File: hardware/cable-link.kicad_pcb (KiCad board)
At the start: 4 copper layers, 50 x 50 mm, 58 parts, among them J1 USB_C_Receptacle_USB2.0, J2 Conn_01x02, J3 GBA-LINK, J4 SWD, Q1 BSS138, Q2 BSS138, Q3 BSS138, Q4 BSS138, U1 NCP1117-3.3_SOT223, U2 RP2040, U3 ATECC608A-MAHDA, U4 W25Q128JVS, Y1 12mhz

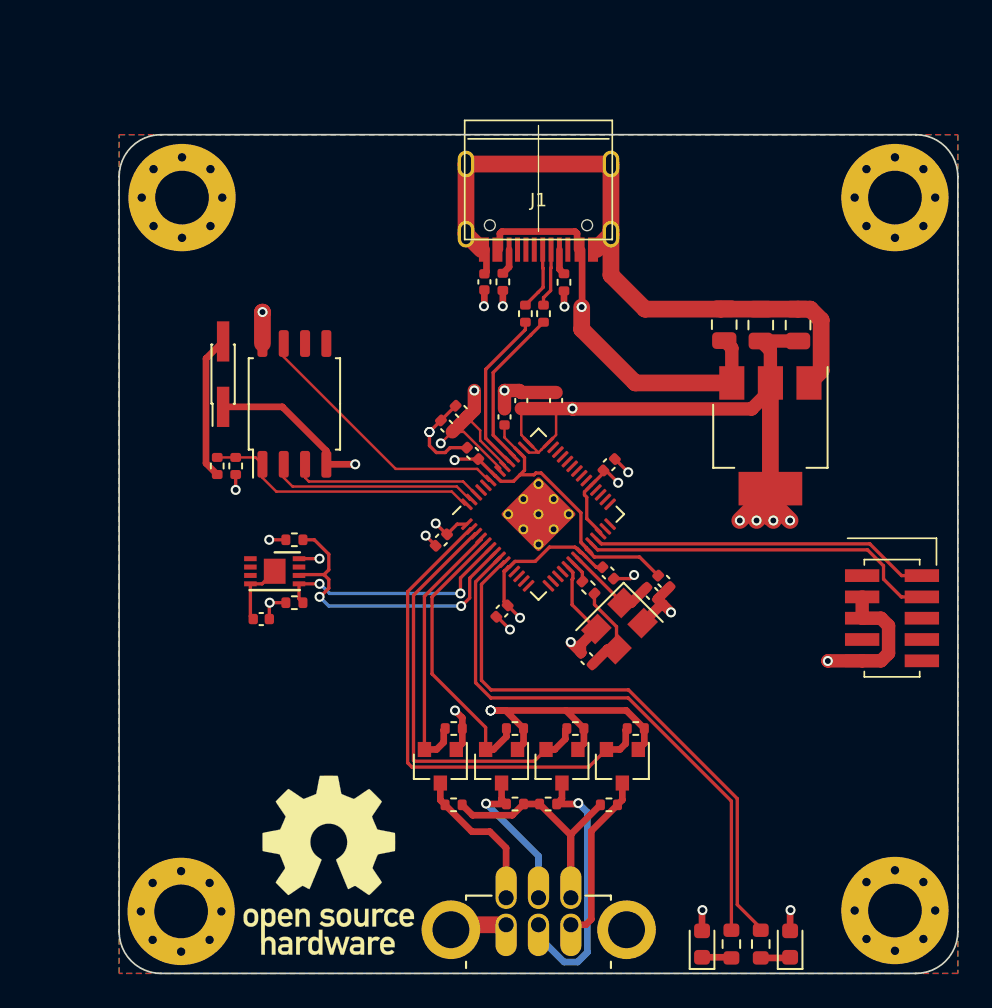
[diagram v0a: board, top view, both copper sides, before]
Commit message: Hardware Rev. C
Redesigned the board yet again. Order placed w/ JLCPCB.
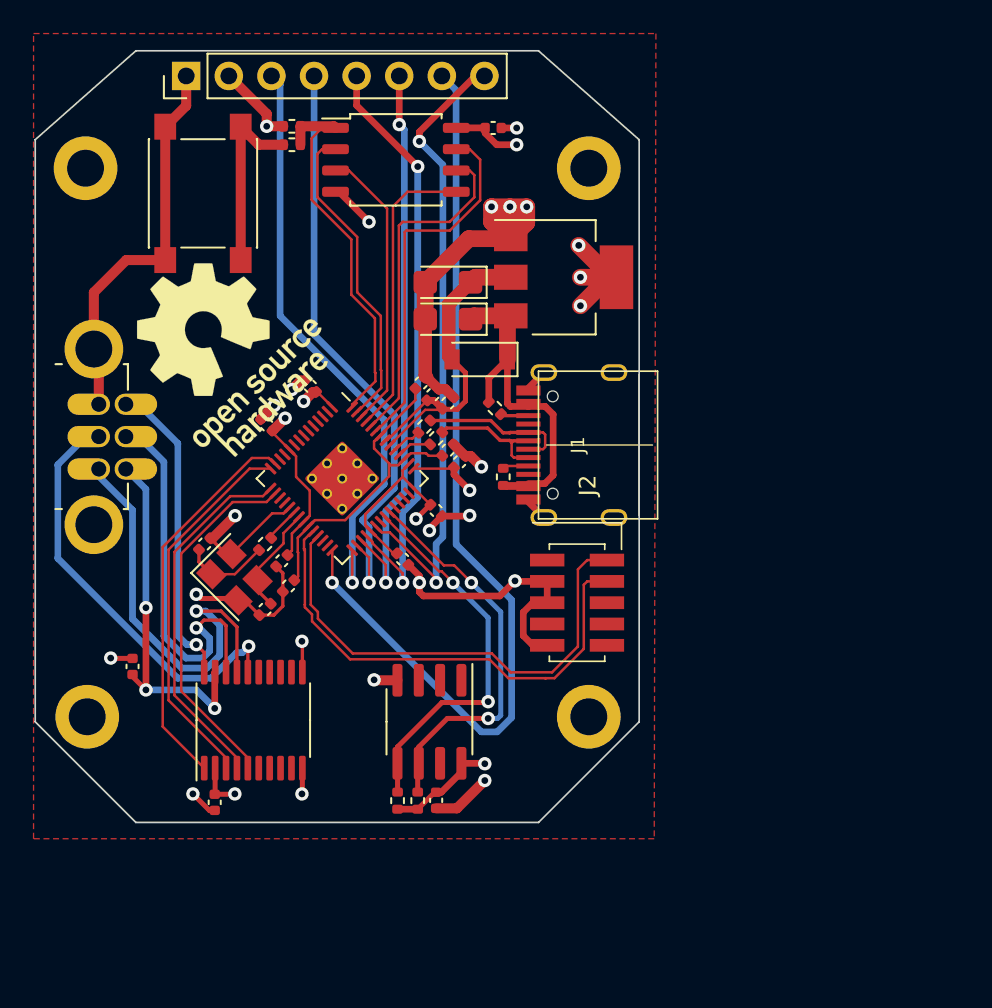
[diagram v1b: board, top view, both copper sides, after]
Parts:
- removed D2: RED, LED_SMD:LED_0603_1608Metric
- removed the G*** at (44.4, 45.0)
- removed Q1, Q2, Q3, Q4: BSS138, Package_TO_SOT_SMD:SOT-23
- removed R10, R11, R12, R13, R14, R15, R16, R17, R18, R19: 10k, Resistor_SMD:R_0402_1005Metric
- added C19: 100n, Capacitor_SMD:C_0402_1005Metric, F.Cu at (20.8, 51.7)
- added SW1: USB_BOOT, Button_Switch_SMD:SW_Push_1P1T_NO_6x6mm_H9.5mm, F.Cu at (25.0, 23.5)
- added U5: TXS0108EPW, Package_SO:TSSOP-20_4.4x6.5mm_P0.65mm, F.Cu at (28.0, 54.9)
- C1: value 12p -> 100n
- C11, C5, C9: value 10u -> 100n; footprint Capacitor_SMD:C_0805_2012Metric -> Capacitor_SMD:C_0402_1005Metric
- C15: value 100n -> 1u
- C16, C17: value 100n -> 10u; footprint Capacitor_SMD:C_0402_1005Metric -> Capacitor_Tantalum_SMD:CP_EIA-3216-18_Kemet-A
- C2: value 12p -> 22p
- C3: value 100n -> 22p
- C6: value 2u2 -> 1u
- C7: value 1u -> 100n
- D1: value RED -> B5819W; footprint LED_SMD:LED_0603_1608Metric -> Diode_SMD:D_SOD-123
- H1, H2, H3, H4: footprint MountingHole:MountingHole_3.2mm_M3_Pad_Via -> MountingHole:MountingHole_2.2mm_M2_DIN965_Pad
- J1: value USB_C_Receptacle_USB2.0 -> USB; footprint Connector_USB_C_JLCPCB:TYPE-C-31-M-12 -> Connector_USBC:TYPE-C-31-M-12
- J2: value Conn_01x02 -> SWD; footprint Connector_PinHeader_1.27mm:PinHeader_2x01_P1.27mm_Vertical_SMD -> Connector_SWD:20021221-00010C4LF
- J4: value SWD -> GC9A01; footprint Connector_SWD:20021221-00010C4LF -> Connector_PinHeader_2.54mm:PinHeader_1x08_P2.54mm_Vertical
- R2: value 5.11k -> 1k
- R3: value 5.11k -> DNF
- R4, R5: value 470 -> 56k; footprint Resistor_SMD:R_0603_1608Metric -> Resistor_SMD:R_0402_1005Metric
- R6, R7: value 27 -> 10k
- R8: value 1k -> 27
- R9: value DNF -> 27
- U1: value NCP1117-3.3_SOT223 -> ATECC608A-SSHDA; footprint Package_TO_SOT_SMD:SOT-223-3_TabPin2 -> Package_SO:SOIC-8_3.9x4.9mm_P1.27mm
- U2: value RP2040 -> W25Q128JVS; footprint rp2048:RP2040-QFN-56 -> Package_SO:SOIC-8_5.23x5.23mm_P1.27mm
- U3: value ATECC608A-MAHDA -> RP2040; footprint Package_DFN_QFN:DFN-8-1EP_3x2mm_P0.5mm_EP1.3x1.5mm -> MCU_RaspberryPi_RP2040:RP2040-QFN-56
- U4: value W25Q128JVS -> AMS1117-3.3; footprint Package_SO:SOIC-8_5.23x5.23mm_P1.27mm -> Package_TO_SOT_SMD:SOT-223-3_TabPin2
- moved J4 53.1 mm to (24.0, 16.5), turned to 90 degrees
- moved H3 49.5 mm to (18.1, 54.7)
- moved D1 39.5 mm to (41.5, 33.4), turned to 180 degrees
- moved J3 36.9 mm to (20.4, 38.0), turned to 270 degrees
- moved C18 34.9 mm to (25.7, 59.8), turned to 270 degrees
- moved R5 34.9 mm to (42.4, 36.3), turned to 315 degrees
- moved C11 33.8 mm to (29.7, 45.4), turned to 225 degrees
- moved R4 31.8 mm to (42.9, 40.4), turned to 90 degrees
- moved G*** 31.6 mm to (26.0, 32.6), turned to 45 degrees
- moved C5 30.3 mm to (30.1, 46.9), turned to 225 degrees
- moved R6 30.0 mm to (36.6, 59.7), turned to 90 degrees
- moved R7 30.0 mm to (37.8, 59.7), turned to 90 degrees
- moved C1 29.3 mm to (42.3, 19.6), turned to 0 degrees
- moved H4 26.9 mm to (48.0, 54.7)
- moved U1 26.5 mm to (38.5, 55.0)
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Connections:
- C1 pad 1: /XOUT -> +3V3
- C16 pad 1: +3V3 -> /VBUS
- C3 pad 1: +1V1 -> /XOUT
- C4 pad 1: +1V1 -> +3V3
- C5 pad 1: /VBUS -> +1V1
- C6 pad 1: GND -> +1V1
- C6 pad 2: +1V1 -> GND
- C7 pad 1: GND -> +1V1
- C7 pad 2: +3V3 -> GND
- D1 pad 1: Net-(D1-Pad1) -> /VBUS
- J1 pad A6: /USB_D+ -> /USB_CONN_D+
- J1 pad A7: /USB_D- -> /USB_CONN_D-
- J1 pad A8: (no net) -> Net-(J1-PadA8)
- J1 pad B6: /USB_D+ -> /USB_CONN_D+
- J1 pad B7: /USB_D- -> /USB_CONN_D-
- J1 pad B8: (no net) -> Net-(J1-PadB8)
- J2 pad 1: GND -> Net-(J2-Pad1)
- J2 pad 2: /~USB_BOOT -> /SWD
- J3 pad 2: /GB_SO -> /GBA_SO
- J3 pad 3: /GB_SI -> /GBA_SI
- J3 pad 4: /GB_SD -> /GBA_SD
- J3 pad 5: /GB_SC -> /GBA_SC
- J4 pad 1: (no net) -> GND
- J4 pad 2: /SWD -> +3V3
- J4 pad 3: GND -> /SPI0_SCLK
- J4 pad 4: /SWCLK -> /SPI0_MOSI
- J4 pad 5: GND -> /LCD_RST
- J4 pad 6: (no net) -> /LCD_DC
- J4 pad 7: (no net) -> /LCD_CS
- J4 pad 8: (no net) -> /LCD_BLK
- R2 pad 1: Net-(J1-PadB5) -> /QSPI_SS
- R2 pad 2: GND -> /~USB_BOOT
- R3 pad 1: GND -> +3V3
- R3 pad 2: Net-(J1-PadA5) -> /QSPI_SS
- R4 pad 1: /LED0 -> /VBUS
- R4 pad 2: Net-(D1-Pad1) -> Net-(J1-PadA5)
- R5 pad 1: /LED1 -> /VBUS
- R5 pad 2: Net-(D2-Pad1) -> Net-(J1-PadB5)
- R6 pad 1: /USB_D+ -> +3V3
- R6 pad 2: /MCU_USB_D+ -> /I2C0_SDA
- R7 pad 1: /USB_D- -> +3V3
- R7 pad 2: /MCU_USB_D- -> /I2C0_SCL
- R8 pad 1: /QSPI_SS -> /USB_CONN_D+
- R8 pad 2: /~USB_BOOT -> /USB_D+
- R9 pad 1: +3V3 -> /USB_CONN_D-
- R9 pad 2: /QSPI_SS -> /USB_D-
- U1 pad 1: GND -> (no net)
- U1 pad 2: +3V3 -> (no net)
- U1 pad 3: /VBUS -> (no net)
- U2 pad 1: +3V3 -> /QSPI_SS
- U2 pad 2: /SPI0_RX -> /QSPI_SD1
- U2 pad 3: /SPI0_CSN -> /QSPI_SD2
- U2 pad 4: /SPI0_SCK -> GND
- U2 pad 5: /SPI0_TX -> /QSPI_SD0
- U2 pad 6: /I2C0_SDA -> /QSPI_SCLK
- U2 pad 7: /I2C0_SCL -> /QSPI_SD3
- U2 pad 8: /LED1 -> +3V3
- U3 pad 1: (no net) -> +3V3
- U3 pad 2: (no net) -> Net-(U3-Pad2)
- U3 pad 3: (no net) -> Net-(U3-Pad3)
- U3 pad 4: GND -> Net-(U3-Pad4)
- U3 pad 5: /I2C0_SDA -> Net-(U3-Pad5)
- U3 pad 6: /I2C0_SCL -> Net-(U3-Pad6)
- U3 pad 7: (no net) -> Net-(U3-Pad7)
- U3 pad 8: +3V3 -> Net-(U3-Pad8)
- U3 pad 9: GND -> Net-(U3-Pad9)
- U4 pad 1: /QSPI_SS -> GND
- U4 pad 2: /QSPI_SD1 -> +3V3
- U4 pad 3: /QSPI_SD2 -> /VBUS
- Y1 pad 1: /XOUT -> Net-(C2-Pad1)
- Y1 pad 3: Net-(C2-Pad1) -> /XOUT
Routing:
- net /LCD_CS: track 0.00 -> 56.6 mm, vias 0 -> 1
- net /LCD_BLK: track 0.00 -> 38.0 mm, vias 0 -> 2
- net /LCD_RST: track 0.00 -> 35.8 mm, vias 0 -> 2
- net /SPI0_SCLK: track 0.00 -> 35.7 mm, vias 0 -> 1
- net /SPI0_MOSI: track 0.00 -> 35.6 mm, vias 0 -> 1
- net /LED1: track 34.4 -> 0.00 mm
- net /LED0: track 34.3 -> 0.00 mm
- net /LCD_DC: track 0.00 -> 33.9 mm, vias 0 -> 2
- net /SPI0_RX: track 30.2 -> 0.00 mm
- net +3V3: track 104.6 -> 76.2 mm, vias 21 -> 12
- net /GBA_SO: track 0.00 -> 25.6 mm, vias 0 -> 1
- net /GBA_SD: track 0.00 -> 25.4 mm, vias 0 -> 1
- net /SPI0_CSN: track 25.4 -> 0.00 mm
- net /GBA_SI: track 0.00 -> 23.4 mm, vias 0 -> 1
- net /SPI1_SCLK: track 0.00 -> 23.3 mm
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- added copper zone on In1.Cu, net +3V3
- added copper zone on In2.Cu, net GND
- removed copper zone on B.Cu, net +3V3
- removed copper zone on In2.Cu, net +3V3
- removed copper zone on In1.Cu, net GND
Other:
- board size 50 x 50 mm -> 36 x 46 mm
- net class Default: clearance 0.15 -> 0.2; trace_width 0.15 -> 0.25; via_dia 0.6 -> 0.8; via_drill 0.35 -> 0.4
- net class USB_DIFF added: clearance 0.15, trace_width 0.15, via_dia 0.6, via_drill 0.35
- rule trace_clearance: 0.15 -> 0.2
- rule trace_min: 0 -> 0.15
